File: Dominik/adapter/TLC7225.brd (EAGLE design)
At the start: 18.8 x 32 mm, 2 parts

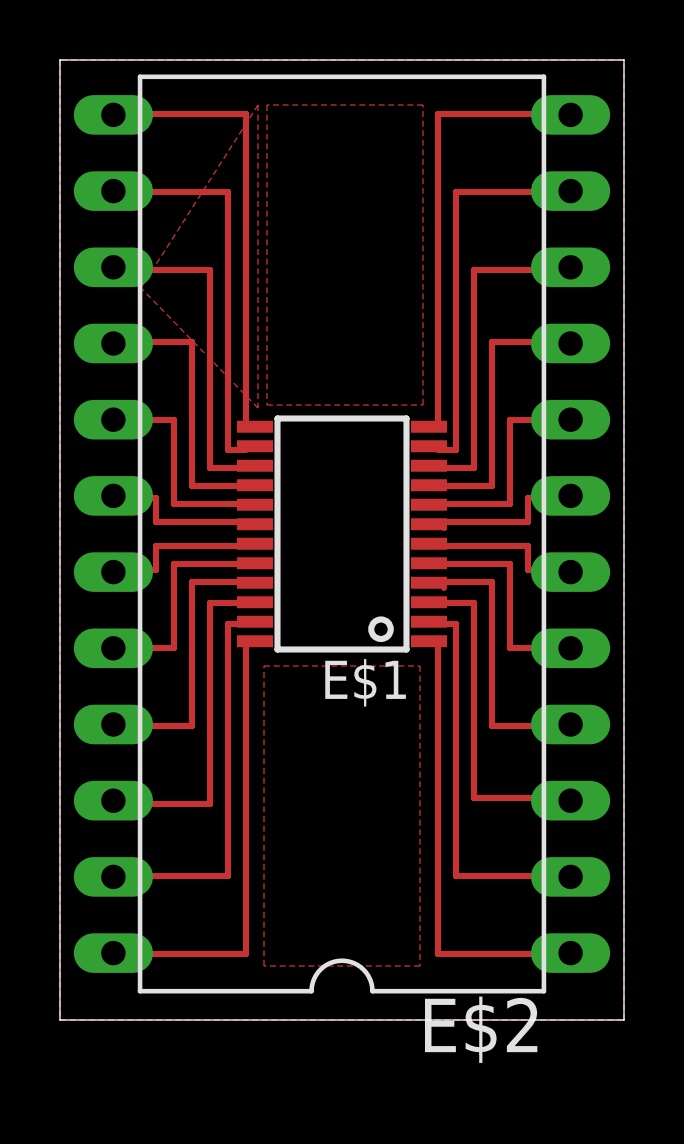
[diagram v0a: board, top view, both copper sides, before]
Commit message: added tictactoe design
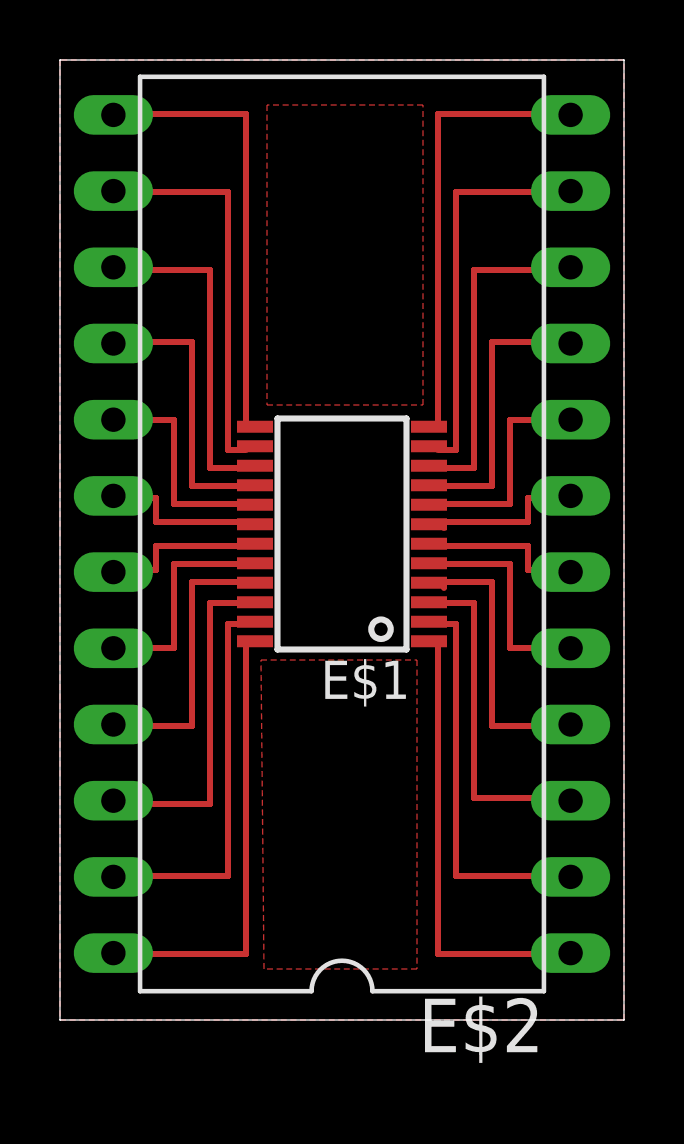
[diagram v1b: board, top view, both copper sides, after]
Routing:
- removed copper zone on layer 1, net S$14
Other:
- board text added: "A"
- board text added: "A-"
- board text added: "B"
- board text added: "C"
- board text added: "D"
- board text added: "D0"
- board text added: "D1"
- board text added: "D2"
- board text added: "D3"
- board text added: "D4"
- board text added: "D5"
- board text added: "D6"
- board text added: "D7"
- board text added: "RB"
- board text added: "RC"
- board text added: "V+"
- board text removed: "AGND"
- board text removed: "DB0"
- board text removed: "DB1"
- board text removed: "DB2"
- board text removed: "DB3"
- board text removed: "DB4"
- board text removed: "DB5"
- board text removed: "DB6"
- board text removed: "DB7"
- board text removed: "OUTA"
- board text removed: "OUTB"
- board text removed: "OUTC"
- board text removed: "OUTD"
- board text removed: "REFB"
- board text removed: "REFC"
- board text removed: "VDD"
- board text removed: "VSS"
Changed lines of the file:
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@@
 <wire x1="26.4" y1="72.8" x2="7.6" y2="72.8" width="0" layer="20"/>
 <wire x1="7.6" y1="72.8" x2="7.6" y2="40.8" width="0" layer="20"/>
-<text x="19.6" y="65.4" size="0.65" layer="41" font="vector" ratio="20" rot="R180" align="top-left">VDD</text>
-<text x="19.6" y="68" size="0.6" layer="41" font="vector" ratio="20" align="bottom-right">OUTD</text>
-<text x="19.7" y="70.6" size="0.65" layer="41" font="vector" ratio="20" align="bottom-right">OUTC</text>
-<text x="19.6" y="63" size="0.65" layer="41" font="vector" ratio="20" align="bottom-right">REFC</text>
-<text x="16.9" y="63" size="0.65" layer="41" font="vector" ratio="20" align="bottom-right">REFB</text>
-<text x="16.3" y="65.4" size="0.65" layer="41" font="vector" ratio="20" align="bottom-right">VSS</text>
-<text x="16.9" y="68" size="0.65" layer="41" font="vector" ratio="20" align="bottom-right">OUTA</text>
-<text x="16.9" y="70.6" size="0.65" layer="41" font="vector" ratio="20" align="bottom-right">OUTB</text>
-<text x="16.3" y="42.7" size="0.65" layer="41" font="vector" ratio="20" align="bottom-right">DB4</text>
-<text x="16.3" y="45.3" size="0.65" layer="41" font="vector" ratio="20" align="bottom-right">DB5</text>
-<text x="16.3" y="47.7" size="0.65" layer="41" font="vector" ratio="20" align="bottom-right">DB6</text>
-<text x="16.3" y="50.3" size="0.65" layer="41" font="vector" ratio="20" align="bottom-right">DB7</text>
-<text x="16.9" y="61.4" size="0.65" layer="41" font="vector" ratio="20" align="bottom-right">AGND</text>
-<text x="19.6" y="61.4" size="0.65" layer="41" font="vector" ratio="20" align="bottom-right">A0</text>
-<text x="19.6" y="42.7" size="0.65" layer="41" font="vector" ratio="20" align="bottom-right">DB3</text>
-<text x="19.6" y="45.3" size="0.65" layer="41" font="vector" ratio="20" align="bottom-right">DB2</text>
-<text x="19.6" y="47.7" size="0.65" layer="41" font="vector" ratio="20" align="bottom-right">DB1</text>
-<text x="19.6" y="50.3" size="0.65" layer="41" font="vector" ratio="20" align="bottom-right">DB0</text>
-<text x="19.6" y="51.9" size="0.65" layer="41" font="vector" ratio="20" align="bottom-right">WR</text>
+<text x="19.8" y="61.3" size="1" layer="41" font="vector" ratio="20" align="bottom-right">A0</text>
+<text x="19.7" y="51.8" size="1" layer="41" font="vector" ratio="20" align="bottom-right">WR</text>
 <text x="16.9" y="51.9" size="0.65" layer="41" font="vector" ratio="20" align="bottom-right">LDAC</text>
+<text x="14.5" y="70.3" size="1" layer="41" font="vector" ratio="20">B</text>
+<text x="14.5" y="68" size="1" layer="41" font="vector" ratio="20">A</text>
+<text x="19.8" y="70.3" size="1" layer="41" font="vector" ratio="20" align="bottom-right">C</text>
+<text x="19.8" y="68" size="1" layer="41" font="vector" ratio="20" align="bottom-right">D</text>
+<text x="14.5" y="61.3" size="1" layer="41" font="vector" ratio="20">A-</text>
+<text x="14.5" y="62.8" size="1" layer="41" font="vector" ratio="20">RB</text>
+<text x="19.8" y="62.8" size="1" layer="41" font="vector" ratio="20" align="bottom-right">RC</text>
+<text x="14.4" y="47.5" size="1" layer="41" font="vector" ratio="20">D6</text>
+<text x="14.3" y="50.1" size="1" layer="41" font="vector" ratio="20">D7</text>
+<text x="14.4" y="45.1" size="1" layer="41" font="vector" ratio="20">D5</text>
+<text x="14.4" y="42.5" size="1" layer="41" font="vector" ratio="20">D4</text>
+<text x="19.7" y="50.1" size="1" layer="41" font="vector" ratio="20" align="bottom-right">D0</text>
+<text x="19.7" y="47.5" size="1" layer="41" font="vector" ratio="20" align="bottom-right">D1</text>
+<text x="19.7" y="45.1" size="1" layer="41" font="vector" ratio="20" align="bottom-right">D2</text>
+<text x="19.7" y="42.5" size="1" layer="41" font="vector" ratio="20" align="bottom-right">D3</text>
+<text x="19.8" y="65.2" size="1" layer="41" font="vector" ratio="20" align="bottom-right">V+</text>
 </plain>
 <attributes>
@@
 </polygon>
 </signal>
-<signal name="S$14">
-<polygon width="0" layer="1" orphans="yes">
-<vertex x="14.2" y="71.3"/>
-<vertex x="14.2" y="61.2"/>
-<vertex x="10.3" y="65.2"/>
-</polygon>
-</signal>
 <signal name="S$15">
 <polygon width="0" layer="1" orphans="yes">
-<vertex x="14.4" y="52.6"/>
-<vertex x="19.6" y="52.6"/>
-<vertex x="19.6" y="42.6"/>
-<vertex x="14.4" y="42.6"/>
+<vertex x="14.3" y="52.8"/>
+<vertex x="19.5" y="52.8"/>
+<vertex x="19.5" y="42.5"/>
+<vertex x="14.4" y="42.5"/>
 </polygon>
 </signal>
